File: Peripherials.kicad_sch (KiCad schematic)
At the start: 25 parts, among them J12 USB_C_Receptacle_USB2.0_14P, J14 IDC_Cable_02x08, J15 Conn_01x02_Pin, J18 Micro_SD_Card, Q2 NMOS, U12 USBLC6-2P6, U2 RV-3028-C7

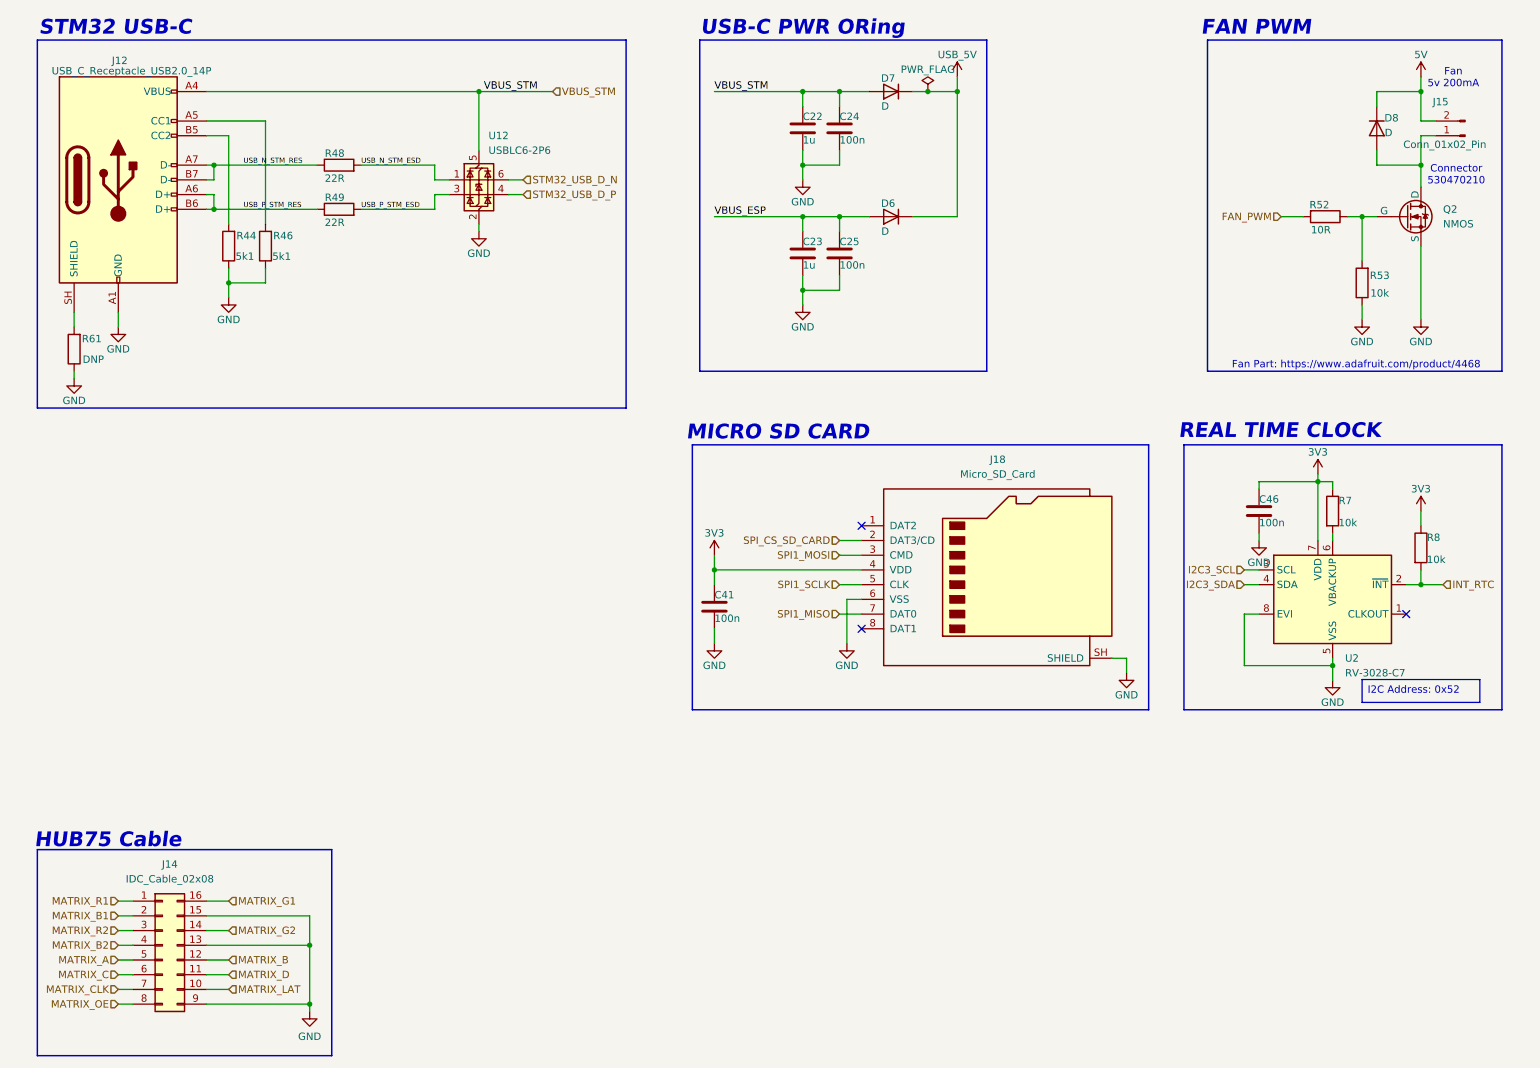
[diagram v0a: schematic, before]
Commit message: Update Peripherials.kicad_sch
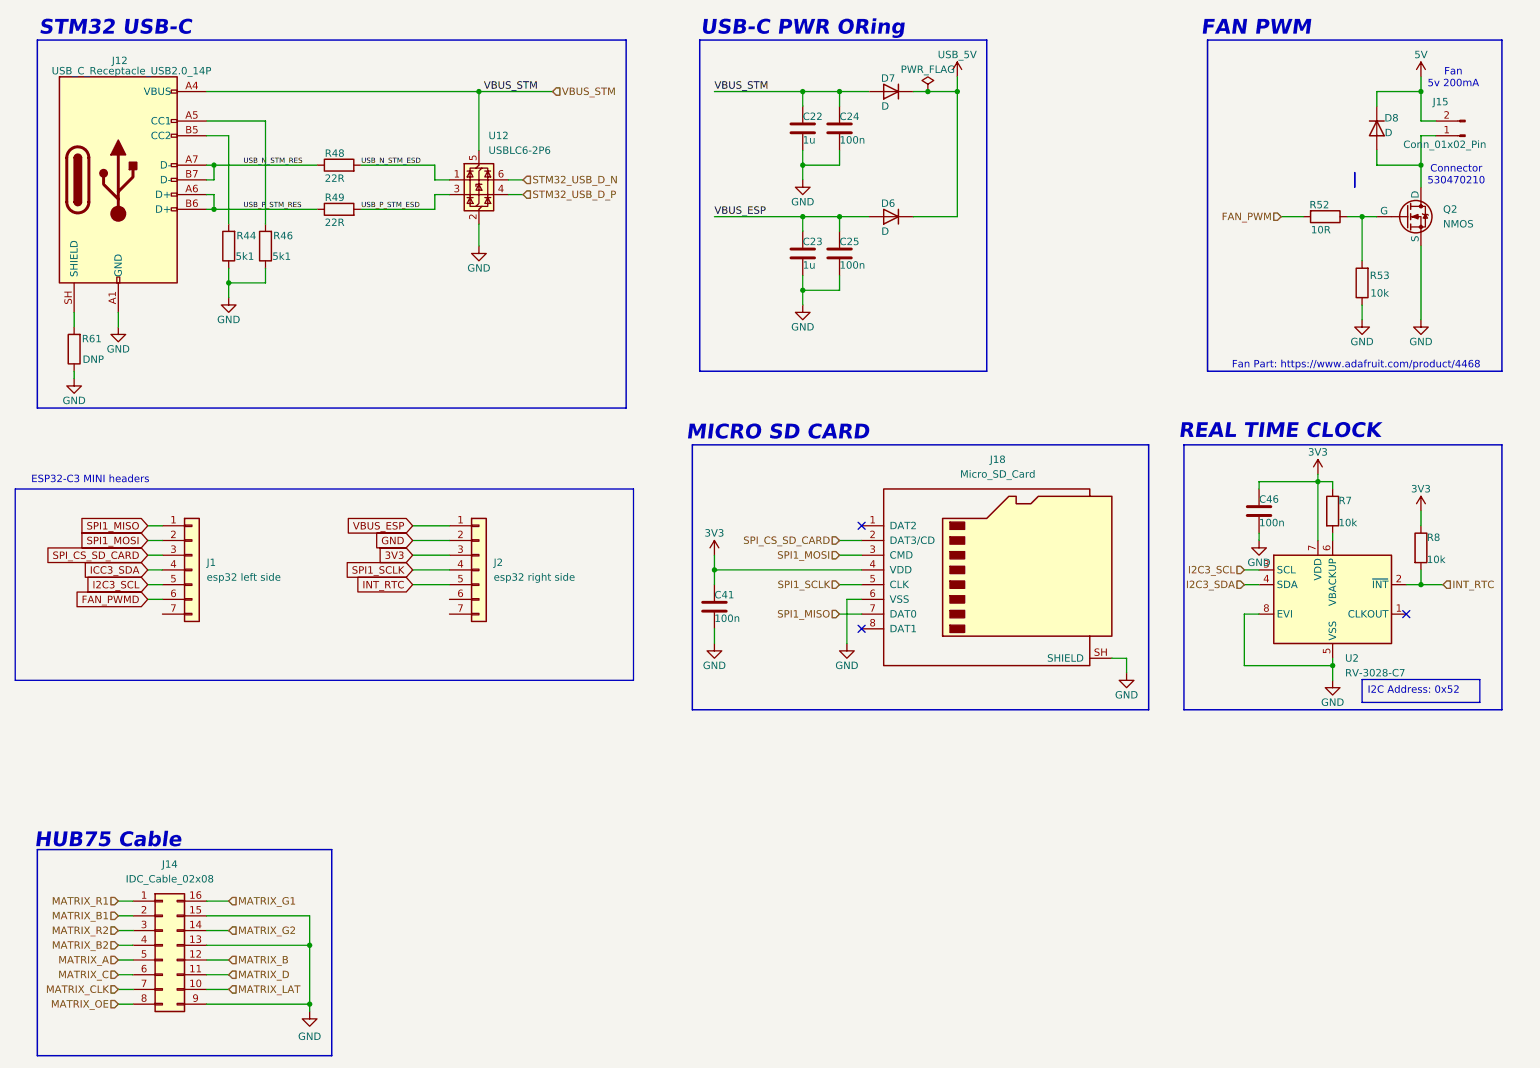
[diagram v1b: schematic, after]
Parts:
- added J1: esp32 left side, symbol Connector_Generic:Conn_01x07
- added J2: esp32 right side, symbol Connector_Generic:Conn_01x07
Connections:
- net 3V3: now also J2.3 (Pin_3)
- net GND: now also J2.2 (Pin_2)
- net I2C3_SCL: now also J1.5 (Pin_5)
- net INT_RTC: now also J2.5 (Pin_5)
- net SPI1_MISO: now also J1.1 (Pin_1)
- net SPI1_MOSI: now also J1.2 (Pin_2)
- net SPI1_SCLK: now also J2.4 (Pin_4)
- net SPI_CS_SD_CARD: now also J1.3 (Pin_3)
- net VBUS_ESP: now also J2.1 (Pin_1)
- new net FAN_PWMD: J1.6 (Pin_6)
- new net ICC3_SDA: J1.4 (Pin_4)
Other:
- note added: "ESP32-C3 MINI headers"
